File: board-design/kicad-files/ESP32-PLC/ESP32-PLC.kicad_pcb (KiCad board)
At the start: 2 copper layers, 58.1 x 172.1 mm, 159 parts, among them J1 640456-3, J2 Conn_ARM_JTAG_SWD_10, J3 302-S101, J4 Conn_02x05_Odd_Even, J5 Conn_02x10_Odd_Even, J6 RJ45_Wuerth_7499010121A, J7 SF53S006VCBR2000, Q1 BC817, Q2 BC817, Q3 BC817, Q4 BC817, U1 BD48ExxG, U2 ESP32-WROVER-E, U3 LAN8720A, U4 EC21, U5 TXS0108EPW, U6 TXS0108EPW, U7 MCP7940N-xSN, Y1 Q25MHz/20ppm/3.2x2.5mm (FL250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

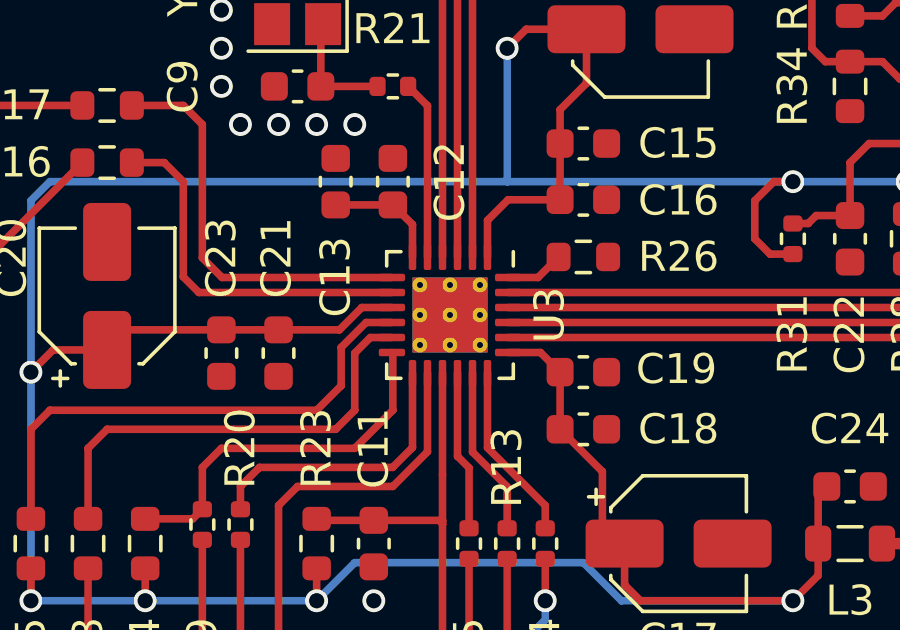
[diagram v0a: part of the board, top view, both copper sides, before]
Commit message: [Final report]
Added 3D models.

Signed-off-by: Nicolae-Andrei Vasile <vasilenicolaeandrei@gmail.com>
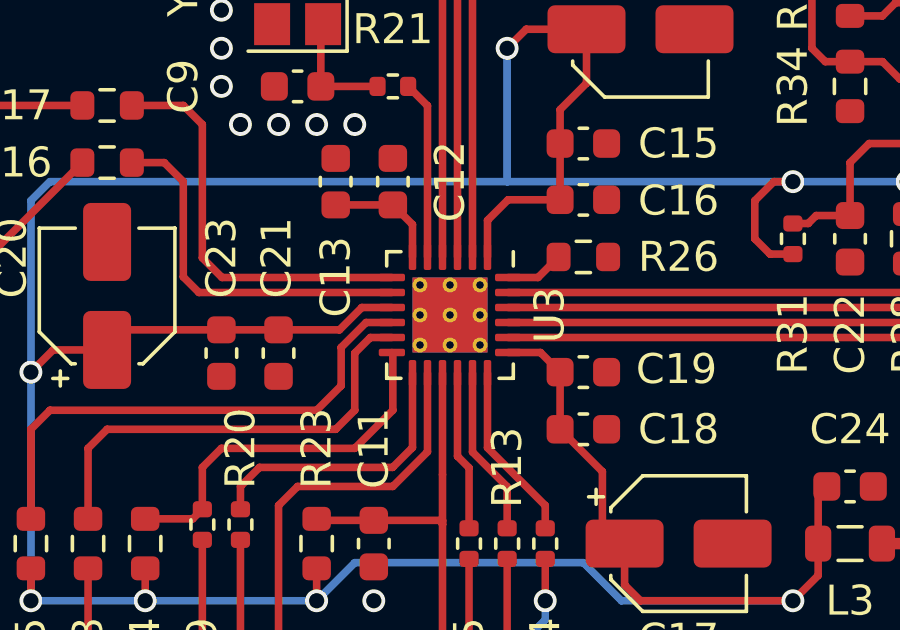
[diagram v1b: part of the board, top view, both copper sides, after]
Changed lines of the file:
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@@
     (pad "4" thru_hole circle locked (at 6.5 4.5 90) (size 2.2 2.2) (drill 1.2) (layers "*.Cu" "*.Mask")
       (net 2 "GND") (pintype "passive"))
+    (model "${KIPRJMOD}/1825910_6.3dshapes/1825910-6.step"
+      (offset (xyz 3.302 -2.286 0))
+      (scale (xyz 1 1 1))
+      (rotate (xyz -90 0 0))
+    )
   )
   (footprint "Inductor_SMD:L_0805_2012Metric" locked (layer "F.Cu")
@@
     (pad "24" smd roundrect locked (at -1.25 -1.9375 270) (size 0.25 0.875) (layers "F.Cu" "F.Paste" "F.Mask") (roundrect_rratio 0.25)
       (net 105 "Net-(U3-RBIAS)") (pinfunction "RBIAS") (pintype "passive"))
-    (pad "25" thru_hole circle locked (at -1 -1 270) (size 0.5 0.5) (drill 0.2) (layers "*.Cu")
+    (pad "25" thru_hole circle locked (at -1 -1 270) (size 0.5 0.5) (drill 0.254) (layers "*.Cu")
       (net 2 "GND") (pinfunction "VSS") (pintype "power_in"))
-    (pad "25" thru_hole circle locked (at -1 0 270) (size 0.5 0.5) (drill 0.2) (layers "*.Cu")
+    (pad "25" thru_hole circle locked (at -1 0 270) (size 0.5 0.5) (drill 0.254) (layers "*.Cu")
       (net 2 "GND") (pinfunction "VSS") (pintype "power_in"))
-    (pad "25" thru_hole circle locked (at -1 1 270) (size 0.5 0.5) (drill 0.2) (layers "*.Cu")
+    (pad "25" thru_hole circle locked (at -1 1 270) (size 0.5 0.5) (drill 0.254) (layers "*.Cu")
       (net 2 "GND") (pinfunction "VSS") (pintype "power_in"))
-    (pad "25" thru_hole circle locked (at 0 -1 270) (size 0.5 0.5) (drill 0.2) (layers "*.Cu")
+    (pad "25" thru_hole circle locked (at 0 -1 270) (size 0.5 0.5) (drill 0.254) (layers "*.Cu")
       (net 2 "GND") (pinfunction "VSS") (pintype "power_in"))
-    (pad "25" thru_hole circle locked (at 0 0 270) (size 0.5 0.5) (drill 0.2) (layers "*.Cu")
+    (pad "25" thru_hole circle locked (at 0 0 270) (size 0.5 0.5) (drill 0.254) (layers "*.Cu")
       (net 2 "GND") (pinfunction "VSS") (pintype "power_in"))
     (pad "25" smd rect locked (at 0 0 270) (size 2.5 2.5) (layers "F.Cu" "F.Mask")
@@
     (pad "25" smd rect locked (at 0 0 270) (size 2.5 2.5) (layers "B.Cu")
       (net 2 "GND") (pinfunction "VSS") (pintype "power_in"))
-    (pad "25" thru_hole circle locked (at 0 1 270) (size 0.5 0.5) (drill 0.2) (layers "*.Cu")
+    (pad "25" thru_hole circle locked (at 0 1 270) (size 0.5 0.5) (drill 0.254) (layers "*.Cu")
       (net 2 "GND") (pinfunction "VSS") (pintype "power_in"))
-    (pad "25" thru_hole circle locked (at 1 -1 270) (size 0.5 0.5) (drill 0.2) (layers "*.Cu")
+    (pad "25" thru_hole circle locked (at 1 -1 270) (size 0.5 0.5) (drill 0.254) (layers "*.Cu")
       (net 2 "GND") (pinfunction "VSS") (pintype "power_in"))
-    (pad "25" thru_hole circle locked (at 1 0 270) (size 0.5 0.5) (drill 0.2) (layers "*.Cu")
+    (pad "25" thru_hole circle locked (at 1 0 270) (size 0.5 0.5) (drill 0.254) (layers "*.Cu")
       (net 2 "GND") (pinfunction "VSS") (pintype "power_in"))
-    (pad "25" thru_hole circle locked (at 1 1 270) (size 0.5 0.5) (drill 0.2) (layers "*.Cu")
+    (pad "25" thru_hole circle locked (at 1 1 270) (size 0.5 0.5) (drill 0.254) (layers "*.Cu")
       (net 2 "GND") (pinfunction "VSS") (pintype "power_in"))
     (model "${KICAD6_3DMODEL_DIR}/Package_DFN_QFN.3dshapes/VQFN-24-1EP_4x4mm_P0.5mm_EP2.5x2.5mm.wrl"
@@
     (pad "SH" thru_hole circle locked (at 5.84 12.345 90) (size 2.2 2.2) (drill 1.6) (layers "*.Cu" "*.Mask")
       (net 29 "Earth_Protective") (pintype "passive"))
-    (model "${KICAD6_3DMODEL_DIR}/Connector_RJ.3dshapes/RJ45_Wuerth_7499010121A_Horizontal.wrl"
-      (offset (xyz 0 0 0))
+    (model "${KIPRJMOD}/7499010121A.3dshapes/7499010121A.STEP"
+      (offset (xyz 7.366 -4.572 7.112))
       (scale (xyz 1 1 1))
-      (rotate (xyz 0 0 0))
+      (rotate (xyz 0 0 -90))
     )
   )
@@
       )
     )
+    (model "${KIPRJMOD}/EC21.3dshapes/EC21AFA-512-STD.step"
+      (offset (xyz 0 0 0))
+      (scale (xyz 1 1 1))
+      (rotate (xyz -90 0 0))
+    )
   )
   (footprint "Package_TO_SOT_SMD:SOT-23" locked (layer "F.Cu")
@@
       )
     )
-    (model "${KICAD7_3RD_PARTY}/3dmodels/com_github_espressif_kicad-libraries/espressif.3dshapes/ESP32-WROVER-E.STEP"
-      (offset (xyz -9 -15.7 0))
+    (model "${KIPRJMOD}/ESP32_WROVER_E.3dshapes/ESP32-WROVER-E-N4R8.step"
+      (offset (xyz 0 0 0))
       (scale (xyz 1 1 1))
-      (rotate (xyz 0 0 0))
+      (rotate (xyz -90 0 0))
     )
   )
@@
     (pad "4" thru_hole circle locked (at 6.5 4.5 270) (size 2.2 2.2) (drill 1.2) (layers "*.Cu" "*.Mask")
       (net 2 "GND") (pintype "passive"))
+    (model "${KIPRJMOD}/1825910_6.3dshapes/1825910-6.step"
+      (offset (xyz 3.302 -2.286 0))
+      (scale (xyz 1 1 1))
+      (rotate (xyz -90 0 0))
+    )
   )
   (footprint "Capacitor_SMD:C_0603_1608Metric" locked (layer "F.Cu")
